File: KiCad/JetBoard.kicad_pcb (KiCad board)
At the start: 2 copper layers, 141.2 x 120.8 mm, 84 parts, among them J1 USB_C_Receptacle_USB2.0_16P, J2 Conn_01x02_Socket, SW1 SW_Push, U1 RP2040, U10 STM8S001J3M, U11 RT5715GQW, U12 BQ25185DLHR, U13 TPS2116DRL, U14 TPS2116DRL, U15 TPS2552DRVR, U16 ATGM336H-5N31, U2 W25Q16JVSS, U4 Si5351A-B-GT, U5 TLV61070ADBVR, U7 TPS7A0533PDBZ, U9 TPS2552DRVR, X2 X1G0042110003_C3013793, Y1 12.000MHz-ABM8-272-T3

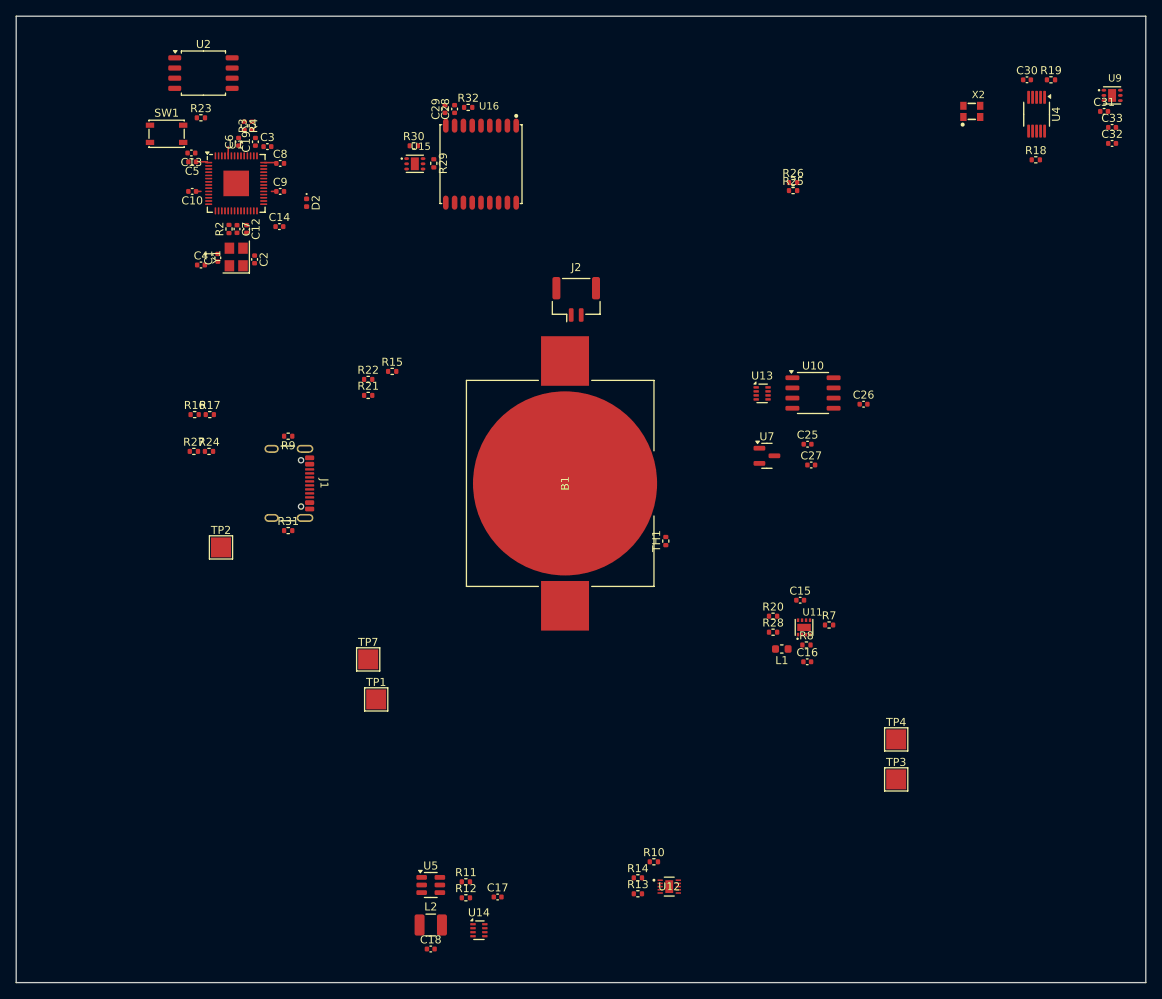
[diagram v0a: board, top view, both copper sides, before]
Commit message: Update schematic and board
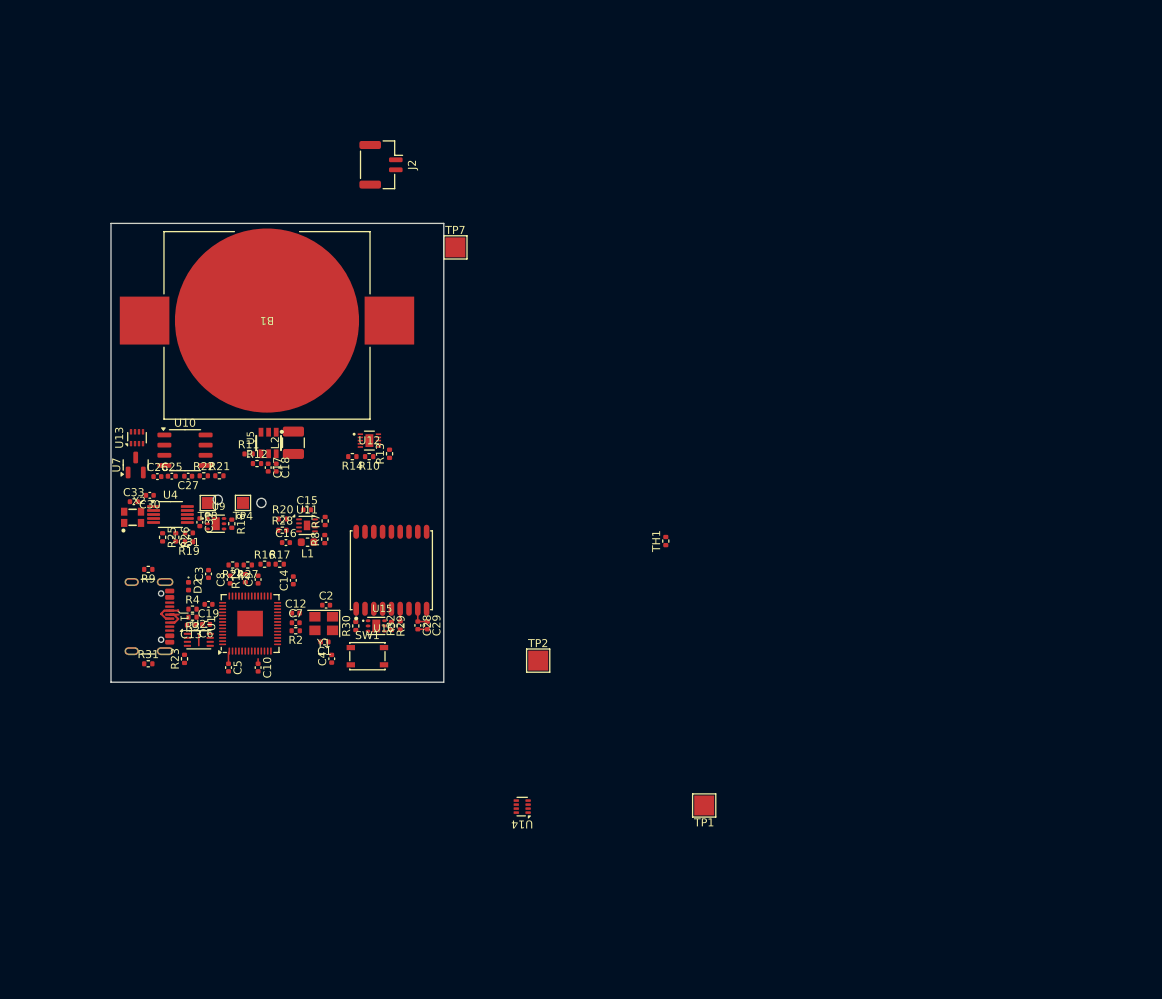
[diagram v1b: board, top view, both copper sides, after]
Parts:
- added H1: MountingHole, MountingHole:ToolingHole_1.152mm, F.Cu at (149.7, 103.4)
- added H2: MountingHole, MountingHole:ToolingHole_1.152mm, F.Cu at (144.2, 103.0)
- J2: footprint Connector_JST:JST_GH_BM02B-GHS-TBT_1x02-1MP_P1.25mm_Vertical -> Connector_JST:JST_GH_SM02B-GHS-TB_1x02-1MP_P1.25mm_Horizontal
- TP3, TP4: footprint TestPoint:TestPoint_Pad_2.5x2.5mm -> TestPoint:TestPoint_Pad_1.5x1.5mm
- U11: footprint JetBoard:WDFN-8_L2.0-W2.0-P0.50-BL-EP -> Package_DFN_QFN:WDFN-8-1EP_2x2mm_P0.5mm_EP0.8x1.2mm
- U2: value W25Q16JVSS -> W25Q16JVUXIQ; footprint Package_SO:SOIC-8_5.3x5.3mm_P1.27mm -> Package_SON:Winbond_USON-8-1EP_3x2mm_P0.5mm_EP0.2x1.6mm
- U5: footprint Package_TO_SOT_SMD:SOT-23-6 -> JetBoard:SOT-23-6_L2.9-W1.6-P0.95-LS2.8-BR
- moved C33 130.9 mm to (133.7, 103.3)
- moved C31 125.9 mm to (140.6, 107.2), turned to 180 degrees
- moved U9 124.2 mm to (143.9, 106.0)
- moved C32 123.5 mm to (141.9, 105.9), turned to -90 degrees
- moved R19 122.2 mm to (140.6, 108.3), turned to 180 degrees
- moved C30 121.3 mm to (135.7, 102.5), turned to 180 degrees
- moved U4 119.3 mm to (138.3, 104.9), turned to 0 degrees
- moved X2 116.5 mm to (133.6, 105.2)
- moved R18 110.3 mm to (145.9, 106.0), turned to -90 degrees
- moved TP3 92.7 mm to (142.9, 103.5), turned to 180 degrees
- moved R25 89.9 mm to (137.3, 107.7), turned to -90 degrees
- moved R26 89.0 mm to (138.9, 107.7), turned to -90 degrees
- moved C26 88.7 mm to (136.7, 100.2)
- moved TP4 86.8 mm to (147.3, 103.4), turned to 180 degrees
- moved C25 79.6 mm to (138.4, 100.1)
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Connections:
- net /jetboard_gnss/3V3_GNSS_EN# renamed /gnss/3V3_GNSS_EN#
- net /jetboard_gnss/GNSS_1PPS renamed /gnss/GNSS_1PPS
- net /jetboard_gnss/GNSS_ANT renamed /gnss/GNSS_ANT
- net /jetboard_gnss/GNSS_RESET# renamed /gnss/GNSS_RESET#
- net /jetboard_gnss/GNSS_UART_RX renamed /gnss/GNSS_UART_RX
- net /jetboard_gnss/GNSS_UART_TX renamed /gnss/GNSS_UART_TX
- C31 pad 1: +3.3V_WSPR -> +3V3_WSPR
- C32 pad 1: +3.3V_WSPR -> +3V3_WSPR
- C33 pad 1: +3.3V_WSPR -> +3V3_WSPR
- J1 pad A6: Net-(J1-D+-PadA6) -> /USB_DP
- J1 pad B6: Net-(J1-D+-PadA6) -> /USB_DP
- R18 pad 1: +3.3V -> +3V3
- U9 pad 1: +3.3V_WSPR -> +3V3_WSPR
- U9 pad 6: +3.3V -> +3V3
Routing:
- net /USB_DP: track 0.00 -> 3.67 mm
- net /USB_DM: track 0.00 -> 3.66 mm
- net +3V3_GNSS: track 0.00 -> 2.80 mm
- net +3V3: track 4.40 -> 2.27 mm
- net VBAT_3V3: track 0.00 -> 1.57 mm
- net GND: track 0.00 -> 1.20 mm
- net /rp2040/QSPI_CLK: track 1.05 -> 0.00 mm
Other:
- board size 141.2 x 120.8 mm -> 41.6 x 57.3 mm
- copper layers 2 -> 4
